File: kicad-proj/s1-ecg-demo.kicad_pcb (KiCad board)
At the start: 4 copper layers, 80.2 x 30.2 mm, 54 parts, among them J1 USB-C-16-Pin, J2 TC2030, J3 Battery Port, J4 Current Probe, J5 ECG_PAD_LA, J6 ECG_PAD_RA, J7 ECG_PAD_RL, U1 AD8233

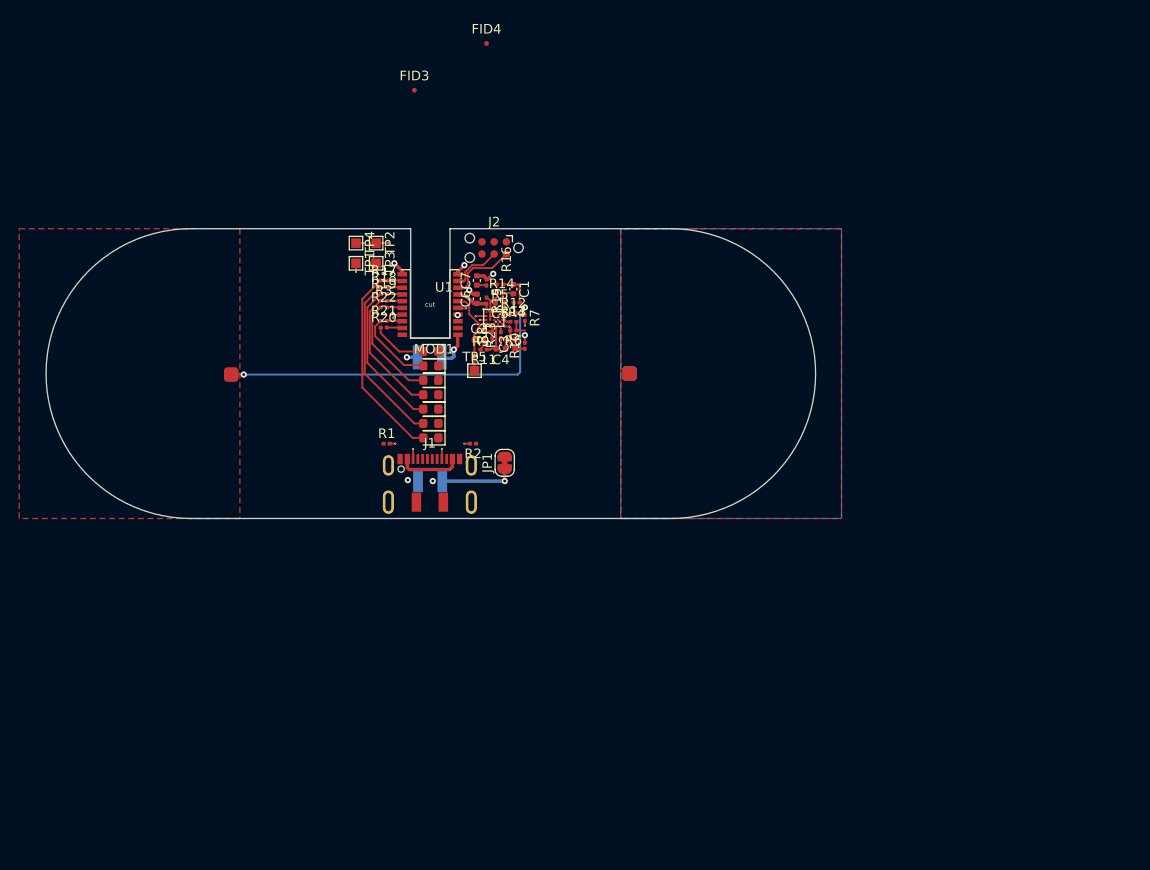
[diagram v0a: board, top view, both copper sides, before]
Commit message: Layout complete, needs checking
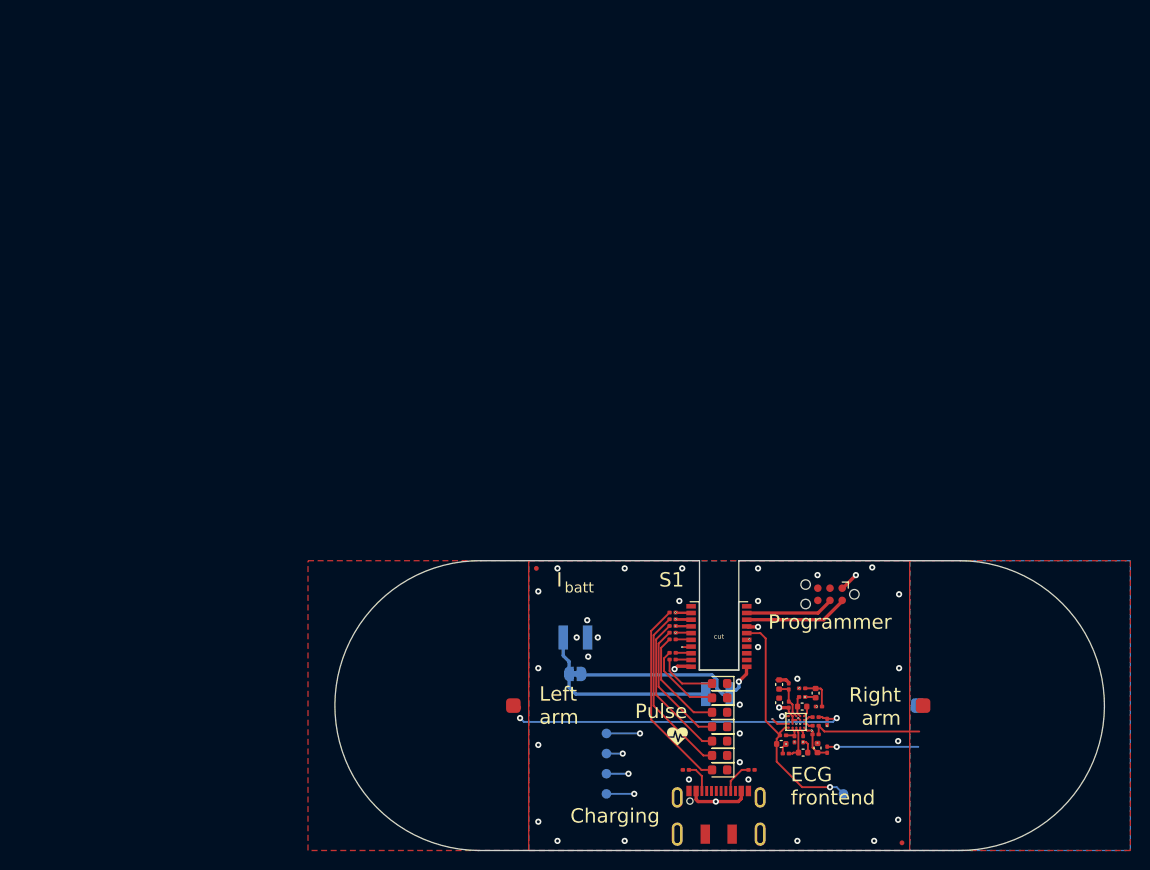
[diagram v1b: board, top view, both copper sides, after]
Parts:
- removed the R14 at (116.3, 60.6)
- removed the R15 at (114.9, 61.4)
- removed the R16 at (114.9, 59.5)
- removed the R23 at (116.4, 65.0)
- removed the R4 at (118.0, 61.6)
- removed the R6 at (117.7, 64.5)
- removed the TP5 at (113.7, 68.7)
- added FID1: Logo, s1-ecg-demo:sw-logo, B.Cu at (110.9, 103.2)
- added FID2: Board title, s1-ecg-demo:title, B.Cu at (117.2, 103.8)
- added FID3: Heartbeat icon, s1-ecg-demo:heartbeat, F.Cu at (134.8, 106.8)
- added R18: 10M, Resistor_SMD:R_0201_0603Metric, F.Cu at (147.8, 102.7)
- added R19: 10M, Resistor_SMD:R_0201_0603Metric, F.Cu at (146.4, 103.5)
- added R2: 200k, Resistor_SMD:R_0201_0603Metric, F.Cu at (147.8, 101.8)
- added R21: 10M, Resistor_SMD:R_0201_0603Metric, F.Cu at (146.4, 101.6)
- added R22: 5.1k, Resistor_SMD:R_0201_0603Metric, F.Cu at (135.7, 110.3)
- added R3: 499k, Resistor_SMD:R_0201_0603Metric, F.Cu at (150.4, 108.2)
- added TP2: D1, TestPoint:TestPoint_Pad_D1.0mm, B.Cu at (127.4, 106.5)
- J1: renamed from J5; value ECG_PAD_LA -> Left arm
- J2: renamed from J6; value ECG_PAD_RA -> Right arm
- J3: renamed from J7; value ECG_PAD_RL -> Right leg
- JP1: moved to B.Cu
- R1: value 5.1k -> 100k
- R10: value 499k -> 1M
- R11: value 1M -> 182k
- R13: value 182k -> 100k
- R5: value 200k -> 10M
- R7: value 10M -> 100k
- R8: value 100k -> 1M
- R9: value 1M -> 10M
- TP1: value Tp -> ECG out; footprint TestPoint:TestPoint_Pad_1.0x1.0mm -> TestPoint:TestPoint_Pad_D1.0mm; moved to B.Cu
- TP3: renamed from TP2; value Tp -> D2; footprint TestPoint:TestPoint_Pad_1.0x1.0mm -> TestPoint:TestPoint_Pad_D1.0mm; moved to B.Cu
- TP4: renamed from TP3; value Tp -> D3; footprint TestPoint:TestPoint_Pad_1.0x1.0mm -> TestPoint:TestPoint_Pad_D1.0mm; moved to B.Cu
- TP5: renamed from TP4; value Tp -> D4; footprint TestPoint:TestPoint_Pad_1.0x1.0mm -> TestPoint:TestPoint_Pad_D1.0mm; moved to B.Cu
- moved FID4 93.5 mm to (158.2, 117.9)
- moved TP1 75.1 mm to (152.1, 112.8), turned to 0 degrees
- moved TP5 63.1 mm to (127.4, 112.8), turned to 90 degrees
- moved TP4 58.4 mm to (127.4, 110.7), turned to 90 degrees
- moved TP3 58.4 mm to (127.4, 108.6), turned to 90 degrees
- moved R5 57.3 mm to (149.2, 106.6)
- moved FID5 54.9 mm to (120.1, 89.3)
- moved R9 54.4 mm to (150.4, 105.3), turned to 270 degrees
- moved R12 53.3 mm to (149.2, 105.7)
- moved R13 53.0 mm to (147.9, 107.1), turned to 90 degrees
- moved R1 52.7 mm to (149.6, 103.7), turned to 180 degrees
- moved C5 52.6 mm to (147.8, 103.7)
- moved C7 52.6 mm to (145.4, 101.4)
- moved C2 52.6 mm to (145.6, 107.6)
- moved C3 52.6 mm to (149.4, 108.0)
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- renumbered FID3 to FID4, FID4 to FID5, J1 to J4, J2 to J5, J4 to J6, J3 to J7, D1 to LED1, D2 to LED2, D3 to LED3, D4 to LED4, D5 to LED5, D6 to LED6, D7 to LED7, R18 to R14, R19 to R15, R20 to R16, R21 to R17, R22 to R20, R2 to R23, R3 to R4, R17 to R6
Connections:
- net /SWDCLK renamed Net-(J5-Pad4)
- net /SWDIO renamed Net-(J5-Pad2)
- J1 pad 1: Net-(J5-Pad1) -> Net-(J1-Pad1)
- J2 pad 1: Net-(J6-Pad1) -> Net-(J2-Pad1)
- J3 pad 1: Net-(J7-Pad1) -> Net-(J3-Pad1)
- J4 pad A5: Net-(J1-PadA5) -> Net-(J4-PadA5)
- R1 pad 1: GND -> Net-(C1-Pad1)
- R1 pad 2: Net-(J1-PadA5) -> Net-(C4-Pad1)
- R10 pad 1: Net-(C3-Pad1) -> Net-(C4-Pad2)
- R10 pad 2: Net-(J7-Pad1) -> Net-(C2-Pad2)
- R11 pad 1: Net-(C4-Pad2) -> Net-(R11-Pad1)
- R11 pad 2: Net-(C2-Pad2) -> Net-(J1-Pad1)
- R12 pad 2: Net-(J5-Pad1) -> Net-(J2-Pad1)
- R13 pad 1: Net-(R13-Pad1) -> Net-(C4-Pad1)
- R13 pad 2: Net-(J6-Pad1) -> Net-(R13-Pad2)
- R5 pad 1: Net-(C1-Pad1) -> Net-(J2-Pad1)
- R5 pad 2: Net-(C2-Pad2) -> Net-(C3-Pad1)
- R7 pad 1: Net-(J5-Pad1) -> Net-(C4-Pad1)
- R7 pad 2: Net-(C3-Pad1) -> Net-(R7-Pad2)
- R8 pad 1: Net-(C4-Pad1) -> Net-(R7-Pad2)
- R8 pad 2: Net-(R8-Pad2) -> /ECG_OUT
- R9 pad 1: Net-(R8-Pad2) -> Net-(J1-Pad1)
- R9 pad 2: /ECG_OUT -> Net-(C3-Pad1)
- TP1 pad 1: /LED1 -> /ECG_OUT
- U1 pad B5: Net-(R12-Pad1) -> Net-(R11-Pad1)
- U1 pad C5: Net-(R13-Pad1) -> Net-(R12-Pad1)
- U1 pad D2: Net-(R8-Pad2) -> Net-(R7-Pad2)
- U1 pad D4: Net-(R23-Pad2) -> Net-(R13-Pad2)
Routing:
- net Net-(J5-Pad1): track 38.1 -> 0.00 mm, vias 2 -> 0
- net Net-(J1-Pad1): track 0.00 -> 35.5 mm, vias 0 -> 2
- net /LED3: track 5.31 -> 23.5 mm
- net /VBUS: track 6.55 -> 23.9 mm, vias 0 -> 2
- net /VBAT: track 3.65 -> 20.3 mm
- net /ECG_OUT: track 9.51 -> 25.5 mm, vias 0 -> 1
- net /LED4: track 9.86 -> 25.2 mm
- net /LED2: track 6.99 -> 21.8 mm
- net Net-(J2-Pad1): track 0.00 -> 11.6 mm
- net Net-(J3-Pad1): track 0.00 -> 9.50 mm, vias 0 -> 1
- net /LED1: track 8.34 -> 17.0 mm
- net /LOD: track 3.56 -> 11.2 mm
- net Net-(J5-Pad4): track 5.06 -> 9.09 mm
- net Net-(J1-PadA5): track 3.68 -> 0.00 mm, vias 2 -> 0
- net Net-(J5-Pad2): track 7.15 -> 10.7 mm
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- added copper zone on In1.Cu, net +1V8
- added copper zone on B.Cu, net GND
- added copper zone on F.Cu, net GND
- added copper zone on In2.Cu, net GND
- added copper zone on F.Cu, net Net-(J1-Pad1)
- added copper zone on F.Cu, net Net-(J2-Pad1)
- added copper zone on B.Cu, net Net-(J3-Pad1)
- removed copper zone on F.Cu, net Net-(J5-Pad1)
- removed copper zone on F.Cu, net Net-(J6-Pad1)
- removed copper zone on B.Cu, net Net-(J7-Pad1)
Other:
- board text added: "Charging"
- board text added: "D1"
- board text added: "D2"
- board text added: "D3"
- board text added: "D4"
- board text added: "ECG frontend"
- board text added: "ECG out"
- board text added: "I"
- board text added: "Left arm"
- board text added: "Programmer"
- board text added: "Pulse"
- board text added: "Right arm"
- board text added: "Right leg"
- board text added: "S1"
- board text added: "batt"
